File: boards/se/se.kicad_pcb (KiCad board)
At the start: 2 copper layers, 97.2 x 56.5 mm, 35 parts, among them J1 SE_PDS, J2 Conn_02x05_Odd_Even, U1 ENC624J600-PT, U3 GAL16V8, U5 LD1117S33TR_SOT223, Y1 25MHz

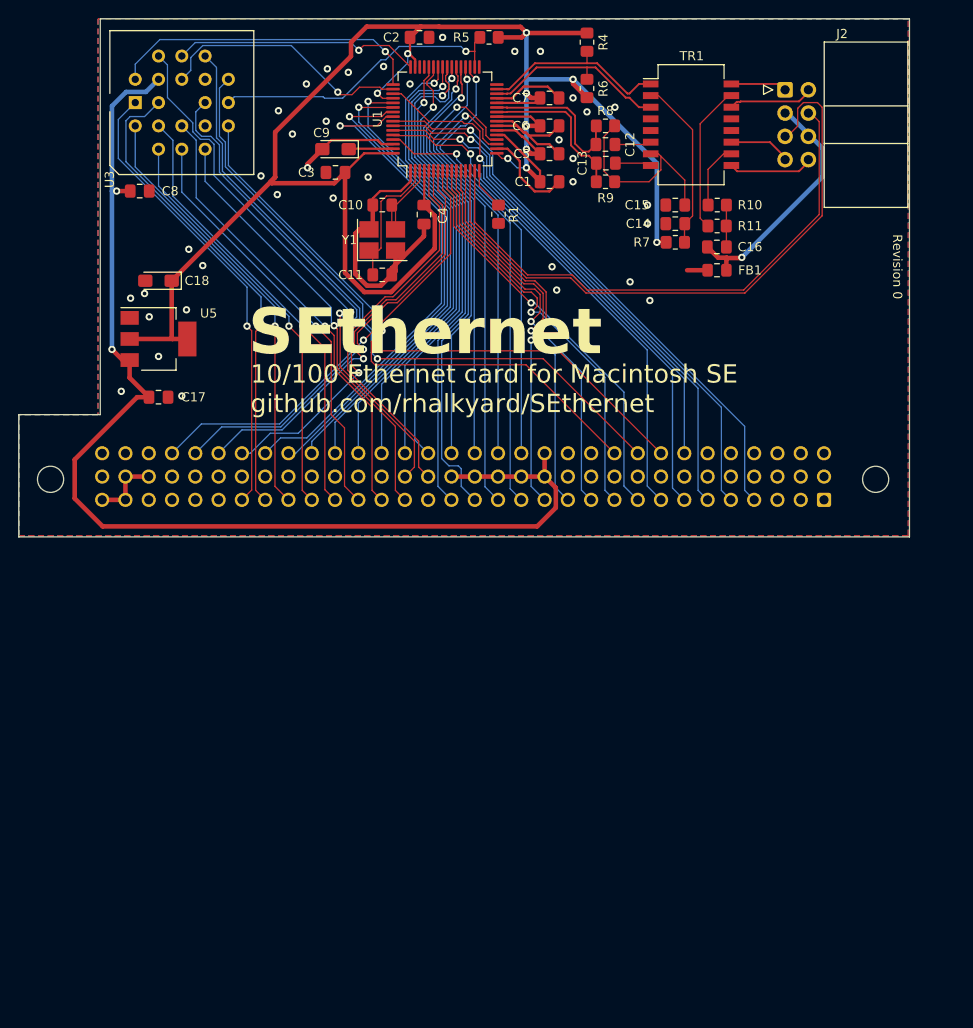
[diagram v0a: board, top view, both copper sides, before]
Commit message: Rev1 hardware
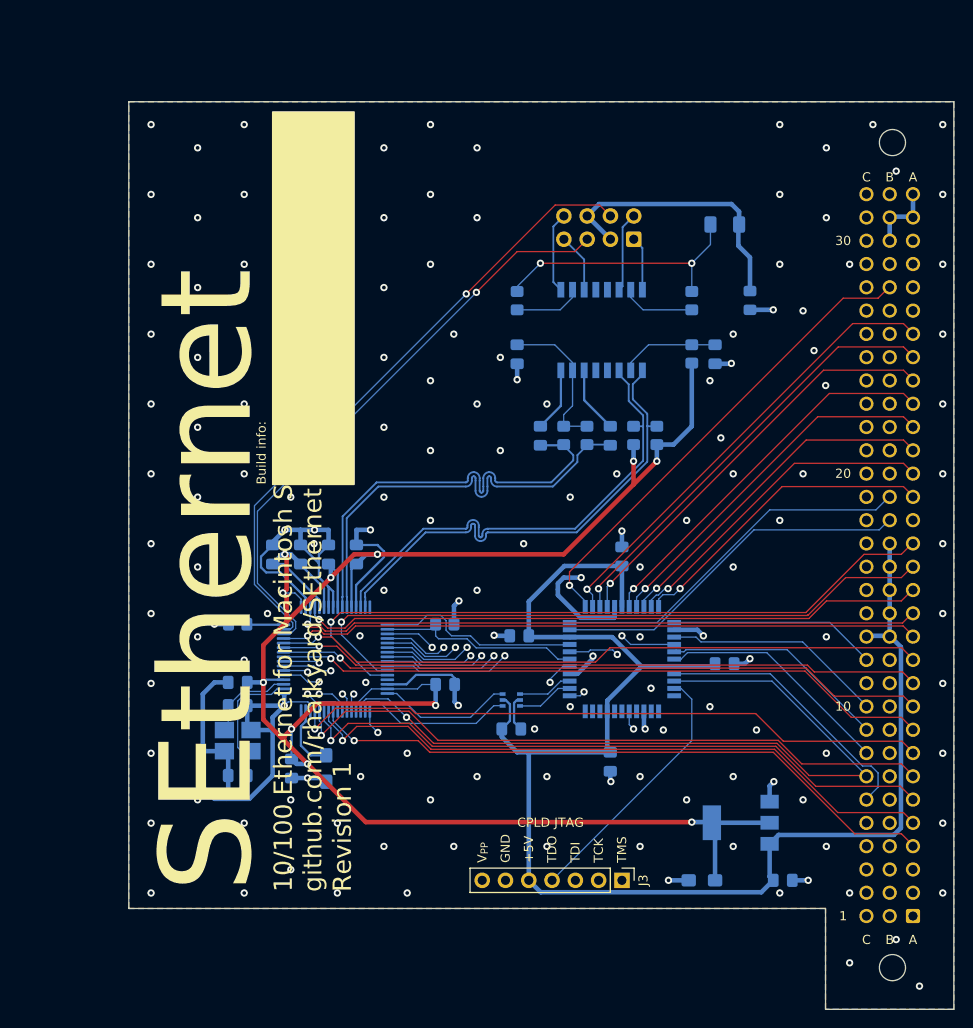
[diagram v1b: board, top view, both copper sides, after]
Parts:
- added C10: 1uF, Capacitor_SMD:C_0805_2012Metric_Pad1.18x1.45mm_HandSolder, B.Cu at (88.9, 77.7)
- added C11: 1uF, Capacitor_SMD:C_0805_2012Metric_Pad1.18x1.45mm_HandSolder, B.Cu at (77.7, 86.4)
- added C12: 1uF, Capacitor_SMD:C_0805_2012Metric_Pad1.18x1.45mm_HandSolder, B.Cu at (100.1, 89.4)
- added C19: 1uF, Capacitor_SMD:C_0805_2012Metric_Pad1.18x1.45mm_HandSolder, B.Cu at (87.6, 100.1)
- added J3: Conn_01x07, Connector_PinHeader_2.54mm:PinHeader_1x07_P2.54mm_Vertical, F.Cu at (88.9, 113.0)
- added U2: ATF1502AS-xAx44, Package_QFP:TQFP-44_10x10mm_P0.8mm, B.Cu at (88.9, 88.9)
- C1: renamed from C16; footprint Capacitor_SMD:C_0805_2012Metric_Pad1.18x1.45mm_HandSolder -> Capacitor_SMD:C_1206_3216Metric_Pad1.33x1.80mm_HandSolder; moved to B.Cu
- C13: renamed from C4; moved to B.Cu
- C14: renamed from C2; moved to B.Cu
- C15: renamed from C10; moved to B.Cu
- C16: renamed from C8; moved to B.Cu
- C17: renamed from C3; moved to B.Cu
- C18: renamed from C9; moved to B.Cu
- C2: renamed from C15; moved to B.Cu
- C20: renamed from C11; moved to B.Cu
- C21: renamed from C18; moved to B.Cu
- C22: renamed from C17; moved to B.Cu
- C3: renamed from C14; moved to B.Cu
- C4: renamed from C13; moved to B.Cu
- C5: renamed from C12; moved to B.Cu
- C6: renamed from C1; moved to B.Cu
- C7: renamed from C5; moved to B.Cu
- C8: renamed from C6; moved to B.Cu
- C9: renamed from C7; moved to B.Cu
- FB1, J2, R6, TR1, U1, Y1: moved to B.Cu
- J1: value SE_PDS -> Macintosh SE PDS Interface; footprint Connector_DIN:DIN41612_C_3x32_Female_Vertical_THT -> PDS-Ethernet:DIN41612_C_3x32_Female_Vertical_THT_Reversed
- R1: renamed from R10; moved to B.Cu
- R2: renamed from R11; moved to B.Cu
- R3: renamed from R7; moved to B.Cu
- R4: renamed from R9; moved to B.Cu
- R5: renamed from R8; moved to B.Cu
- R7: renamed from R4; moved to B.Cu
- R8: renamed from R1; moved to B.Cu
- R9: renamed from R5; moved to B.Cu
- U3: value GAL16V8 -> 74LVC2G17; footprint Package_LCC:PLCC-20_THT-Socket -> Package_TO_SOT_SMD:SOT-363_SC-70-6; moved to B.Cu
- U4: renamed from U5; moved to B.Cu
- moved C21 88.3 mm to (97.6, 113.0)
- moved C22 86.1 mm to (106.4, 113.0)
- moved U4 82.6 mm to (101.9, 106.8), turned to 180 degrees
- moved U3 77.0 mm to (76.8, 93.4), turned to 180 degrees
- moved C16 71.3 mm to (76.8, 96.5)
- moved C14 70.6 mm to (69.6, 91.7)
- moved C18 67.6 mm to (56.6, 100.8), turned to -90 degrees
- moved C17 65.2 mm to (52.9, 100.8), turned to 90 degrees
- moved R9 64.2 mm to (69.6, 85.1)
- moved U1 60.1 mm to (57.7, 88.9), turned to 0 degrees
- moved C15 56.8 mm to (47.0, 94.0), turned to 0 degrees
- moved Y1 56.8 mm to (47.0, 97.8), turned to 180 degrees
- moved C20 56.8 mm to (47.0, 101.6), turned to 180 degrees
- moved C13 54.9 mm to (47.0, 91.4), turned to 0 degrees
- moved C9 54.1 mm to (59.9, 77.5), turned to 90 degrees
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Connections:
- J1 pad b28: unconnected-(J1-~{EXT_DTK}-Padb28) -> ~{EXT_DTK}
- J1 pad c12: unconnected-(J1-~{RESET}-Padc12) -> ~{RESET}
- J1 pad c6: unconnected-(J1-~{DTACK}-Padc6) -> ~{DTACK}
- R9 pad 1: +3.3V -> GND
- U1 pad 33: unconnected-(U1-CLKOUT-Pad33) -> /ETH_CLK
- U1 pad 48: /B1SEL -> /B1SEL'
- U1 pad 49: Net-(U1-~{CS}/CS) -> /ETH_CS
- U1 pad 50: /B0SEL -> /B0SEL'
- U3 pad 1: A23 -> /B1SEL
- U3 pad 2: A22 -> GND
- U3 pad 3: A21 -> /B0SEL
- U3 pad 4: A20 -> /B0SEL'
- U3 pad 5: A19 -> +5V
- U3 pad 6: A18 -> /B1SEL'
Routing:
- net GND: track 76.8 -> 162.7 mm, vias 37 -> 160
- net ~{EXT_DTK}: track 0.00 -> 52.3 mm, vias 0 -> 1
- net ~{UDS}: track 73.5 -> 24.7 mm, vias 1 -> 0
- net ~{LDS}: track 72.6 -> 25.8 mm, vias 1 -> 0
- net ~{AS}: track 63.8 -> 24.1 mm, vias 1 -> 0
- net /CPLD_VPP: track 0.00 -> 36.6 mm, vias 0 -> 1
- net D12: track 43.7 -> 79.7 mm
- net +5V: track 128.5 -> 164.3 mm, vias 2 -> 0
- net D13: track 46.0 -> 80.6 mm
- net Net-(U1-~{CS}/CS): track 34.5 -> 0.00 mm, vias 1 -> 0
- net /TCK: track 0.00 -> 33.8 mm, vias 0 -> 1
- net D14: track 47.7 -> 81.2 mm
- net D15: track 48.8 -> 81.9 mm
- net /TPOUT-: track 21.1 -> 52.7 mm
- net /TPOUT+: track 21.1 -> 52.6 mm
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- added copper zone on In1.Cu, net GND
- added copper zone on In2.Cu, net GND
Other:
- board size 97.2 x 56.5 mm -> 90 x 99 mm
- copper layers 2 -> 4
- board text added: "+5V"
- board text added: "10/100 Ethernet for Macintosh SE github.com/rhalkyard/SEthernet Revision 1"
- board text added: "3"
- board text added: "Build info:"
- board text added: "CPLD JTAG"
- board text added: "GND"
- board text added: "TCK"
- board text added: "TDI"
- board text added: "TDO"
- board text added: "TMS"
- board text added: "V_{PP}"
- board text removed: "10/100 Ethernet card for Macintosh SE github.com/rhalkyard/SEthernet"
- board text removed: "Revision 0"
